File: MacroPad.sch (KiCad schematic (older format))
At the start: 56 parts, among them J1 AVR-ISP-6, SW1 Rotary_Encoder_Switch, SW10 *, SW11 9, SW12 6, SW13 3, SW14 ., SW15 -, SW16 +, SW17 Enter, SW18 SW_Push, SW2 7, SW3 4, SW4 1, SW5 0, SW6 /, SW7 8, SW8 5, SW9 2, U1 ATmega32U4-AU, U2 PRTR5V0U2X, Y1 16Mhz

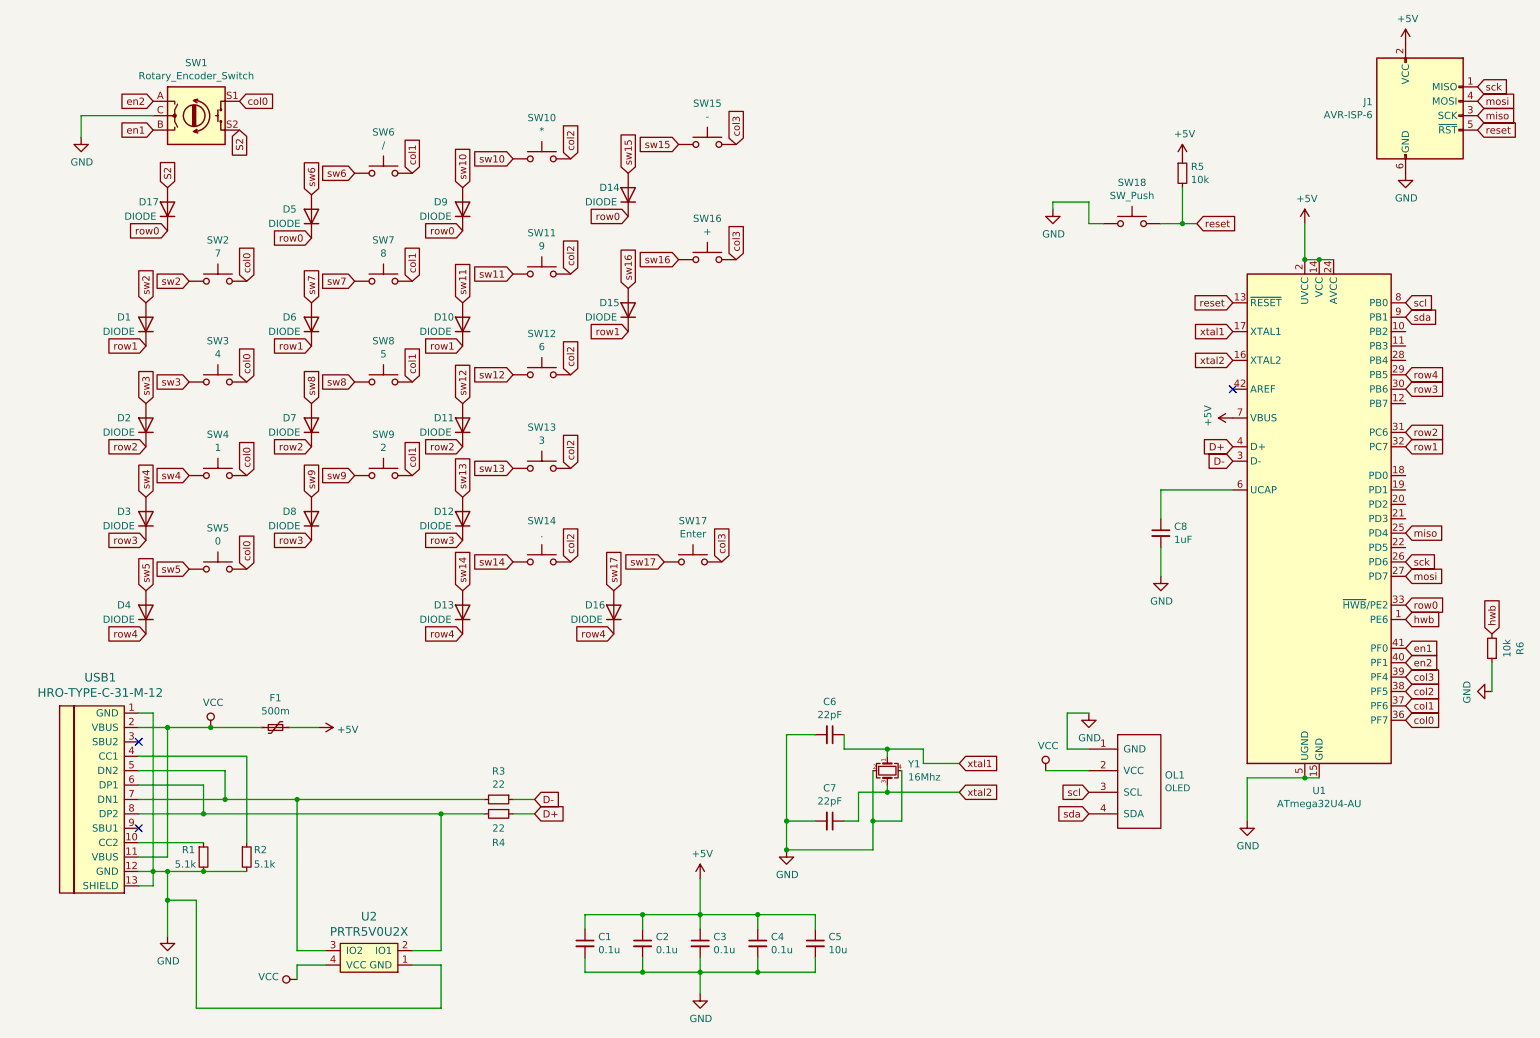
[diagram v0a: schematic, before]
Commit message: cambiando rutas
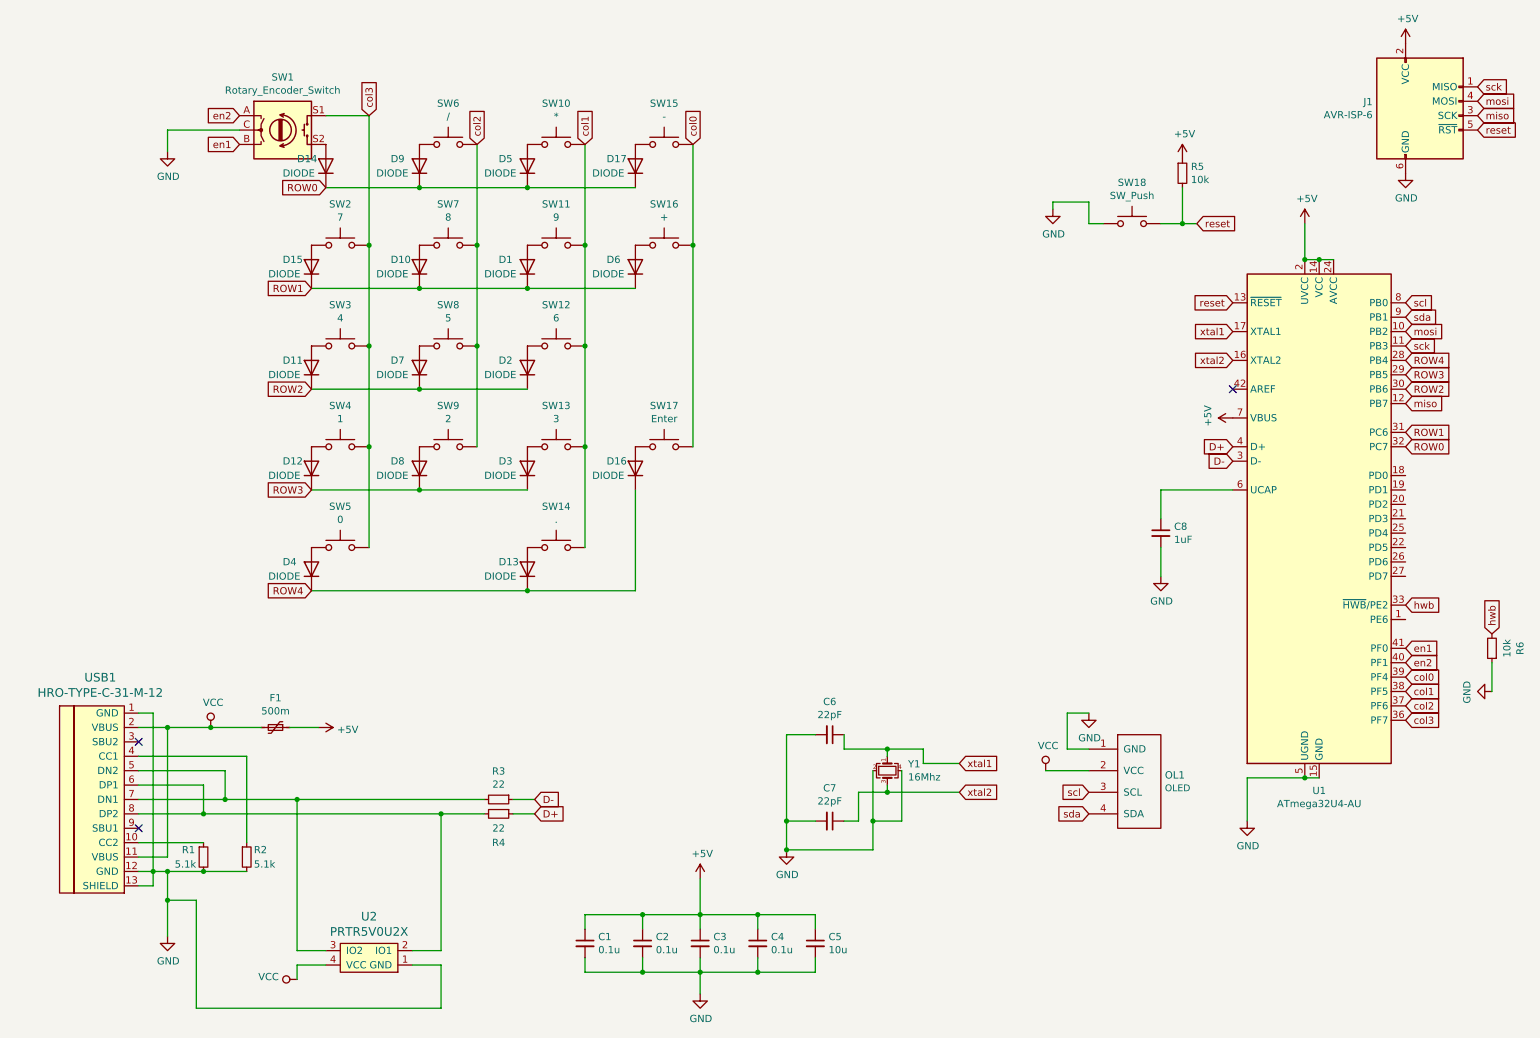
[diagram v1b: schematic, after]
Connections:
- net col0: now also SW15.2, SW16.2, SW17.2, U1.39 (PF4); no longer SW1.S1, SW2.2, SW3.2, SW4.2, SW5.2, U1.36 (PF7)
- net col1: now also SW10.2, SW11.2, SW12.2, SW13.2, SW14.2, U1.38 (PF5); no longer SW6.2, SW7.2, SW8.2, SW9.2, U1.37 (PF6)
- net col2: now also SW6.2, SW7.2, SW8.2, SW9.2, U1.37 (PF6); no longer SW10.2, SW11.2, SW12.2, SW13.2, SW14.2, U1.38 (PF5)
- net col3: now also SW1.S1, SW2.2, SW3.2, SW4.2, SW5.2, U1.36 (PF7); no longer SW15.2, SW16.2, SW17.2, U1.39 (PF4)
- net hwb: now also U1.33 (~HWB~/PE2); no longer U1.1 (PE6)
- net miso: now also U1.12 (PB7); no longer U1.25 (PD4)
- net mosi: now also U1.10 (PB2); no longer U1.27 (PD7)
- net sck: now also U1.11 (PB3); no longer U1.26 (PD6)
- net ROW4: now reaches U1.28 (PB4)
- net ROW4: now also D13.2 (K), D16.2 (K), D4.2 (K)
- net S2: no longer names the net of SW1.S2
- net S2: now also D14.1 (A); no longer D17.1 (A)
- net row0 renamed ROW0
- net ROW0: now also U1.32 (PC7); no longer U1.33 (~HWB~/PE2)
- net row1 renamed ROW1
- net ROW1: now also U1.31 (PC6); no longer U1.32 (PC7)
- net row2 renamed ROW2
- net ROW2: now also U1.30 (PB6); no longer U1.31 (PC6)
- net row3 renamed ROW3
- net ROW3: now also U1.29 (PB5); no longer U1.30 (PB6)
- removed net row4: D13.2 (K), D16.2 (K), D4.2 (K), U1.29 (PB5)
- net sw10: no longer names the net of D9.1 (A)
- net sw10: now also SW6.1; no longer SW10.1
- net sw11: no longer names the net of SW11.1
- net sw11: now also D1.1 (A); no longer D10.1 (A)
- net sw12: no longer names the net of D11.1 (A)
- net sw12: now also SW3.1; no longer SW12.1
- net sw13: no longer names the net of D12.1 (A)
- net sw13: now also SW4.1; no longer SW13.1
- net sw14: no longer names the net of D13.1 (A), SW14.1
- net sw15: no longer names the net of SW15.1
- net sw15: now also D17.1 (A); no longer D14.1 (A)
- net sw16: no longer names the net of D15.1 (A)
- net sw16: now also SW2.1; no longer SW16.1
- net sw17: no longer names the net of D16.1 (A), SW17.1
- removed net sw2: D1.1 (A), SW2.1
- net sw3: no longer names the net of D2.1 (A)
- net sw3: now also SW12.1; no longer SW3.1
- net sw4: no longer names the net of D3.1 (A)
- net sw4: now also SW13.1; no longer SW4.1
- net sw5: no longer names the net of D4.1 (A), SW5.1
- net sw6: no longer names the net of D5.1 (A)
- net sw6: now also SW10.1; no longer SW6.1
- net sw7: no longer names the net of SW7.1
- net sw7: now also D10.1 (A); no longer D6.1 (A)
- net sw8: no longer names the net of D7.1 (A), SW8.1
- net sw9: no longer names the net of D8.1 (A), SW9.1
- new net: D6.1 (A), SW16.1
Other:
- moved on the sheet: D1, D10, D11, D12, D13, D14, D15, D16, D17, D2, D3, D4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
